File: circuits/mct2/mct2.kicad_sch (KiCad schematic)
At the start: 29 parts, among them J1 Bus_M.2_Socket_M, J2 Bus_M.2_Socket_E

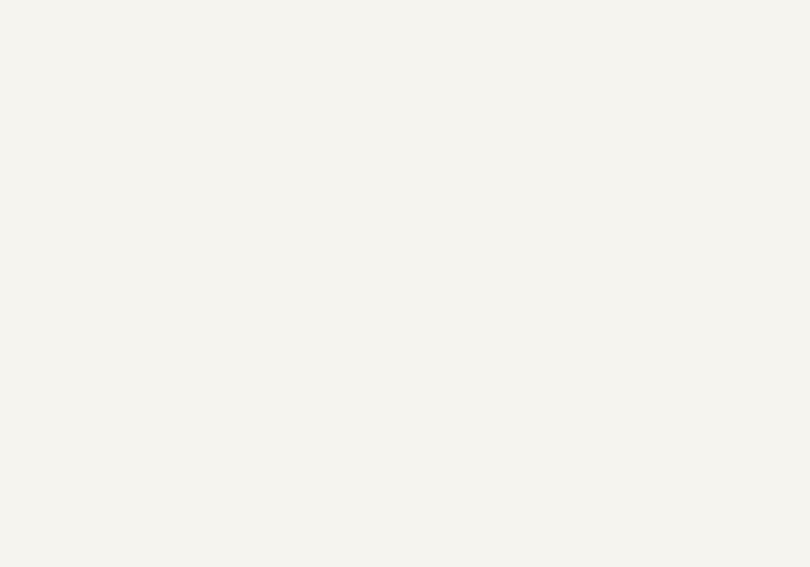
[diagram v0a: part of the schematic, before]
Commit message: Aug 1, 2024
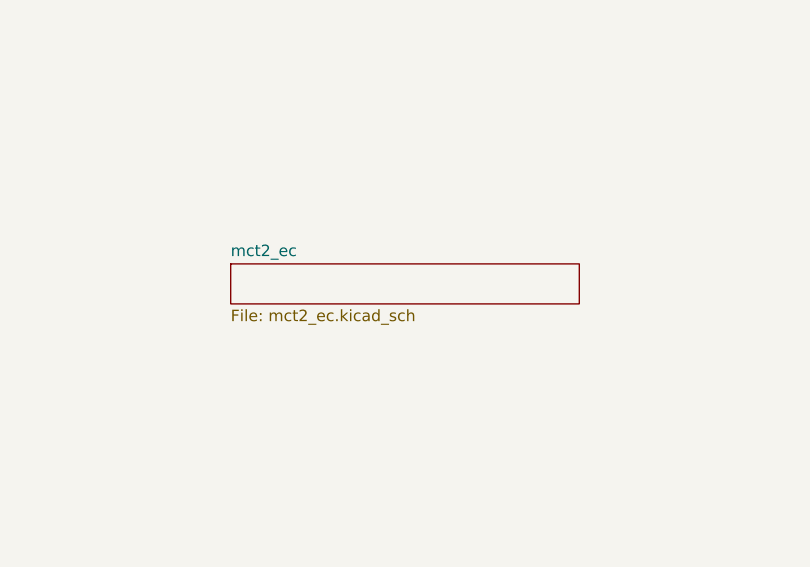
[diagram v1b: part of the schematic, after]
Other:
- added sheet mct2_ec (mct2_ec.kicad_sch)
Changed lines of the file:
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@@
+		)
+	)
+	(sheet
+		(at 931.545 391.16)
+		(size 38.735 4.445)
+		(fields_autoplaced yes)
+		(stroke
+			(width 0.1524)
+			(type solid)
+		)
+		(fill
+			(color 0 0 0 0.0000)
+		)
+		(property "Sheetname" "mct2_ec"
+			(at 931.545 390.4484 0)
+			(effects
+				(font
+					(size 1.27 1.27)
+				)
+				(justify left bottom)
+			)
+		)
+		(property "Sheetfile" "mct2_ec.kicad_sch"
+			(at 931.545 396.1896 0)
+			(effects
+				(font
+					(size 1.27 1.27)
+				)
+				(justify left top)
+			)
+		)
+		(instances
+			(project "mct2"
+				(path "/0917e100-0497-47cd-9e32-3e43ad224d2b"
+					(page "4")
+				)
+			)
 		)
 	)

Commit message: Aug 10, 2024
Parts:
- removed SW?: SW_DIP_x01, symbol Switch:SW_DIP_x01
- added BT?: Battery_Cell, symbol Device:Battery_Cell
- added C? (x8): 220nF, symbol Device:C_Small
- added J?: Conn_01x02, symbol Connector_Generic:Conn_01x02
- added R?: 1K, symbol Device:R_Small
- added R?: 10K, symbol Device:R_Small
- added SW?: CTS 204121ST, symbol Switch:SW_SPDT
- U?: value ~ -> SOIC-8 208mil Socket; footprint (none) -> Package_SO:SOIC-8_5.275x5.275mm_P1.27mm
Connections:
- net GND: now also A1.101 (GND), A1.107 (GND), A1.11 (GND), A1.110 (GND), A1.113 (GND), A1.116 (GND), A1.135 (GND), A1.136 (GND), A1.14 (GND), A1.151 (GND), A1.158 (GND), A1.167 (GND), A1.17 (GND), A1.170 (GND), A1.181 (GND), A1.182 (GND), A1.188 (GND), A1.189 (GND), A1.194 (GND), A1.195 (GND), A1.20 (GND), A1.200 (GND), A1.201 (GND), A1.206 (GND), A1.207 (GND), A1.212 (GND), A1.213 (GND), A1.218 (GND), A1.219 (GND), A1.224 (GND), A1.225 (GND), A1.23 (GND), A1.230 (GND), A1.231 (GND), A1.236 (GND), A1.237 (GND), A1.242 (GND), A1.243 (GND), A1.248 (GND), A1.249 (GND), A1.26 (GND), A1.29 (GND), A1.32 (GND), A1.35 (GND), A1.38 (GND), A1.41 (GND), A1.44 (GND), A1.47 (GND), A1.50 (GND), A1.53 (GND), A1.56 (GND), A1.59 (GND), A1.62 (GND), A1.65 (GND), A1.68 (GND), A1.71 (GND), A1.74 (GND), A1.77 (GND), A1.80 (GND), A1.83 (GND), A1.86 (GND), A1.89 (GND), A1.92 (GND), A1.95 (GND), A1.98 (GND), A1.MP (Mountinge_Pads), J1.1 (GND), J1.15 (GND), J1.21 (GND), J1.27 (GND), J1.3 (GND), J1.33 (GND), J1.39 (GND), J1.45 (GND), J1.51 (GND), J1.57 (GND), J1.71 (GND), J1.73 (GND), J1.75 (GND), J1.9 (GND), BT?.2 (-), R?.2
- net PCIE_REFCLK_E_N: now also A1.90 (REFCLK3-)
- net PCIE_REFCLK_E_P: now also A1.88 (REFCLK3+)
- net PCIE_RX0_E_N: now also A1.30 (HSIO2_RX-)
- net PCIE_RX0_E_P: now also A1.28 (HSIO2_RX+)
- net PCIE_TX0_E_N: now also A1.27 (HSIO2_TX-)
- net PCIE_TX0_E_P: now also A1.25 (HSIO2_TX+)
- net SOM_IO_3V3: now reaches C?.1, C?.1, R?.2, U?. (VCC)
- net SOM_IO_3V3: now also R?.1
- net at A1.133 (~{BIOS_SEL}): now also SW?.2 (B)
- net USB_M2E_P: now reaches J2.3 (USB_D+)
- net USB_M2E_P: now also A1.111 (USB2_P5+)
- net USB_M2E_N: now reaches J2.5 (USB_D-)
- net USB_M2E_N: now also A1.109 (USB2_P5-)
- net USB_CAM_P: now reaches A1.112 (USB2_P6+)
- net USB_CAM_N: now reaches A1.114 (USB2_P6-)
- net at A1.115 (VBAT): now also BT?.1 (+)
- net at A1.137 (UART0_RXD): now also J?.1 (Pin_1)
- net at A1.139 (UART0_TXD): now also J?.2 (Pin_2)
- net VSYS: now reaches A1.250 (VIN), A1.251 (VIN), A1.252 (VIN), A1.253 (VIN), A1.254 (VIN), A1.255 (VIN), A1.256 (VIN), A1.257 (VIN), A1.258 (VIN), A1.259 (VIN), A1.260 (VIN)
- net PCIE_NVME_TX0_P: now reaches A1.37 (HSIO8_TX+)
- net PCIE_NVME_TX0_P: now also C?.1
- net PCIE_NVME_TX0_N: now reaches A1.39 (HSIO8_TX-)
- net PCIE_NVME_TX0_N: now also C?.1
- net PCIE_NVME_RX0_P: now reaches A1.40 (HSIO8_RX+)
- net PCIE_NVME_RX0_P: now also J1.43 (PERp0/SATA-B-)
- net PCIE_NVME_RX0_N: now reaches A1.42 (HSIO8_RX-)
- net PCIE_NVME_RX0_N: now also J1.41 (PERn0/SATA-B+)
- net PCIE_NVME_TX1_P: now reaches A1.43 (HSIO9_TX+)
- net PCIE_NVME_TX1_P: now also C?.1
- net PCIE_NVME_TX1_N: now reaches A1.45 (HSIO9_TX-)
- net PCIE_NVME_TX1_N: now also C?.1
- net PCIE_NVME_RX1_P: now reaches A1.46 (HSIO9_RX+)
- net PCIE_NVME_RX1_P: now also J1.31 (PERp1)
- net PCIE_NVME_RX1_N: now reaches A1.48 (HSIO9_RX-)
- net PCIE_NVME_RX1_N: now also J1.29 (PERn1)
- net PCIE_NVME_TX2_P: now reaches A1.49 (HSIO10_TX+)
- net PCIE_NVME_TX2_P: now also C?.1
- net PCIE_NVME_TX2_N: now reaches A1.51 (HSIO10_TX-)
- net PCIE_NVME_TX2_N: now also C?.1
- net PCIE_NVME_RX2_P: now reaches A1.52 (HSIO10_RX+)
- net PCIE_NVME_RX2_P: now also J1.19 (PERp2)
- net PCIE_NVME_RX2_N: now reaches A1.54 (HSIO10_RX-)
- net PCIE_NVME_RX2_N: now also J1.17 (PERn2)
- net PCIE_NVME_TX3_P: now reaches A1.55 (HSIO11_TX+)
- net PCIE_NVME_TX3_P: now also C?.1
- net PCIE_NVME_TX3_N: now reaches A1.57 (HSIO11_TX-)
- net PCIE_NVME_TX3_N: now also C?.1
- net PCIE_NVME_RX3_P: now reaches A1.58 (HSIO11_RX+)
- net PCIE_NVME_RX3_P: now also J1.7 (PERp3)
- net PCIE_NVME_RX3_N: now reaches A1.60 (HSIO11_RX-)
- net PCIE_NVME_RX3_N: now also J1.5 (PERn3)
- net USB_EXT1_N: now reaches A1.67 (USB2_P1-)
- net USB_EXT1_P: now reaches A1.69 (USB2_P1+)
- net USB_EXT4_P: now reaches A1.70 (USB2_P4+)
- net USB_EXT4_N: now reaches A1.72 (USB2_P4-)
- net USB_EXT2_N: now reaches A1.73 (USB2_P2-)
- net USB_EXT2_P: now reaches A1.75 (USB2_P2+)
- net USB_EXT3_N: now reaches A1.79 (USB2_P3-)
- net USB_EXT3_P: now reaches A1.81 (USB2_P3+)
- net PCIE_NVME_REF_P: now reaches A1.94 (REFCLK4+)
- net PCIE_NVME_REF_P: now also J1.55 (REFCLKp)
- net PCIE_NVME_REF_N: now reaches A1.96 (REFCLK4-)
- net PCIE_NVME_REF_N: now also J1.53 (REFCLKn)
- net PCIE_REFCLK_LAN_P: now reaches A1.97 (REFCLK2+)
- net PCIE_REFCLK_LAN_N: now reaches A1.99 (REFCLK2-)
- net at J1.11 (PETn3): now also C?.2
- net at J1.13 (PETp3): now also C?.2
- net at J1.23 (PETn2): now also C?.2
- net at J1.25 (PETp2): now also C?.2
- net at J1.35 (PETn1): now also C?.2
- net at J1.37 (PETp1): now also C?.2
- net at J1.47 (PETn0/SATA-A-): now also C?.2
- net at J1.49 (PETp0/SATA-A+): now also C?.2
- net SMB_AL renamed SOM_SMB_ALT
- net SMB_CLK renamed SOM_SMB_SCL
- net SMB_D renamed SOM_SMB_SDA
- net TCP_SML_AL renamed SMB3_ALT
- net TCP_SML_CLK renamed SMB3_SCL
- net TCP_SML_D renamed SMB3_SDA
- new net: R?.2, SW?.1 (A)
- new net: R?.1, SW?.3 (C)
- no-connect marks 42 -> 40
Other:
- note removed: "Verify: Should this be pulled low; has a pull-up resistor?"
- moved on the sheet: C?, R?, U?

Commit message: Aug 11, 2024 2
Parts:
- added U?: TPD4EUSB30, Package_TO_SOT_SMD:Texas_DRT-3, symbol mediacow:TPD2EUSB30
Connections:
- net GND: now also J2.1 (GND), J2.18 (GND), J2.33 (GND), J2.39 (GND), J2.45 (GND), J2.51 (GND), J2.57 (GND), J2.63 (GND), J2.69 (GND), J2.7 (GND), J2.75 (GND), U?.3 (GND)
- net USB_M2E_N: now also U?.2 (D1-)
- net USB_M2E_P: now also U?.1 (D1+)
- net SIO_UART_TX: now reaches A1.10 (SIO_UART_TX)
- net SIO_UART_RX: now reaches A1.12 (SIO_UART_RX)
- net TCP1_HPD: now reaches A1.185 (TCP1_HPD)
- net TCP0_HPD: now reaches A1.187 (TCP0_HPD)
- net TCP0_AUX_N: now reaches A1.221 (TCP0_AUX-)
- net TCP0_AUX_P: now reaches A1.223 (TCP0_AUX+)
- net TCP1_AUX_P: now reaches A1.244 (TCP1_AUX+)
- net TCP1_AUX_N: now reaches A1.246 (TCP1_AUX-)
- net PCIE_LAN_TX0_P: now reaches A1.31 (HSIO3_TX+)
- net PCIE_LAN_TX0_N: now reaches A1.33 (HSIO3_TX-)
- net PCIE_LAN_RX0_P: now reaches A1.34 (HSIO3_RX+)
- net PCIE_LAN_RX0_N: now reaches A1.36 (HSIO3_RX-)
- net PCIE_REFCLK_E_N renamed PCIE_M2E_REF_N
- net PCIE_REFCLK_E_P renamed PCIE_M2E_REF_P
- net PCIE_REFCLK_LAN_N renamed PCIE_LAN_REF_N
- net PCIE_REFCLK_LAN_P renamed PCIE_LAN_REF_P
- net PCIE_RX0_E_N renamed PCIE_M2E_RX0_N
- net PCIE_RX0_E_P renamed PCIE_M2E_RX0_P
- net PCIE_TX0_E_N renamed PCIE_M2E_TX0_N
- net PCIE_TX0_E_P renamed PCIE_M2E_TX0_P
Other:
- note added: "CTCL 2021-2024"
- note added: "July 4, 2024 - August 11, 2024"
- note added: "MediaCow Touch 2 - System"
